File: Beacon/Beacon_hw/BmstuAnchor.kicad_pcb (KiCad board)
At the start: 2 copper layers, 62 x 60 mm, 46 parts, among them U1 MCP1700T-3002E/TT

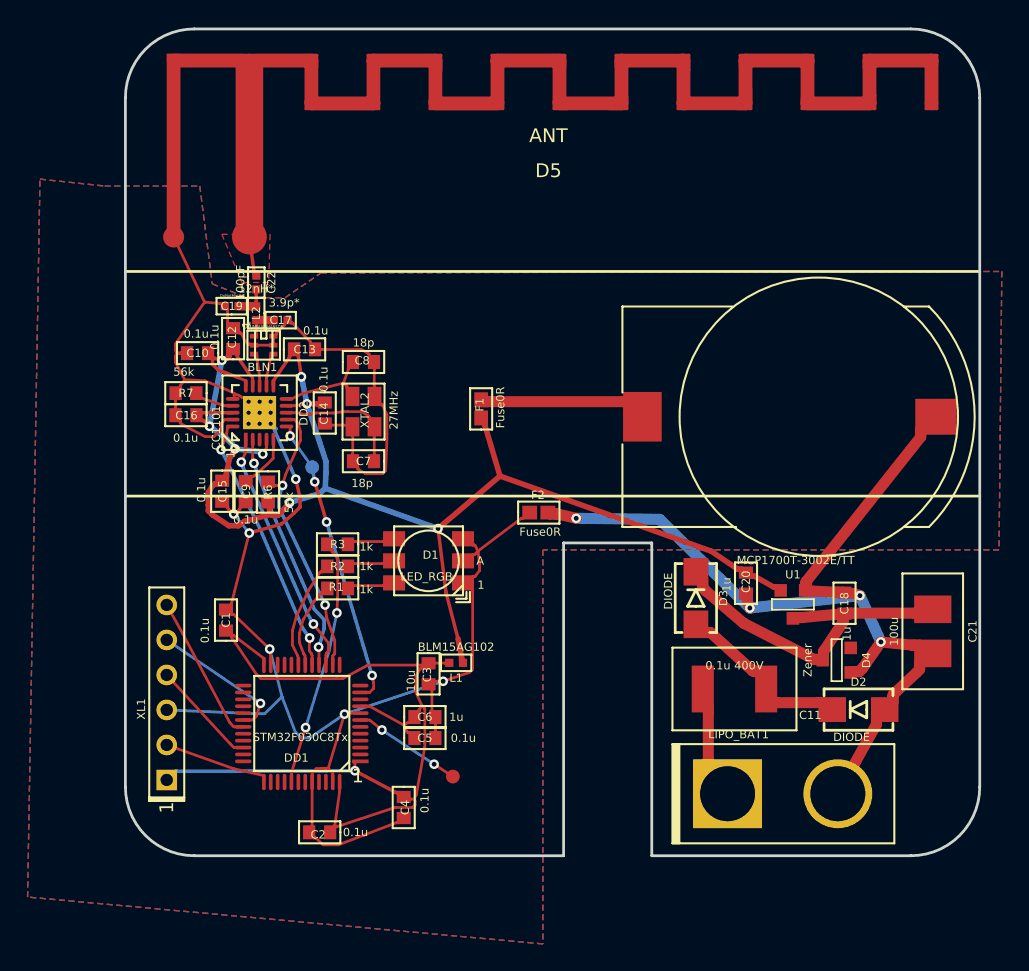
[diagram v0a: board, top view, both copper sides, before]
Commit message: +axp library *beaco pcb upd
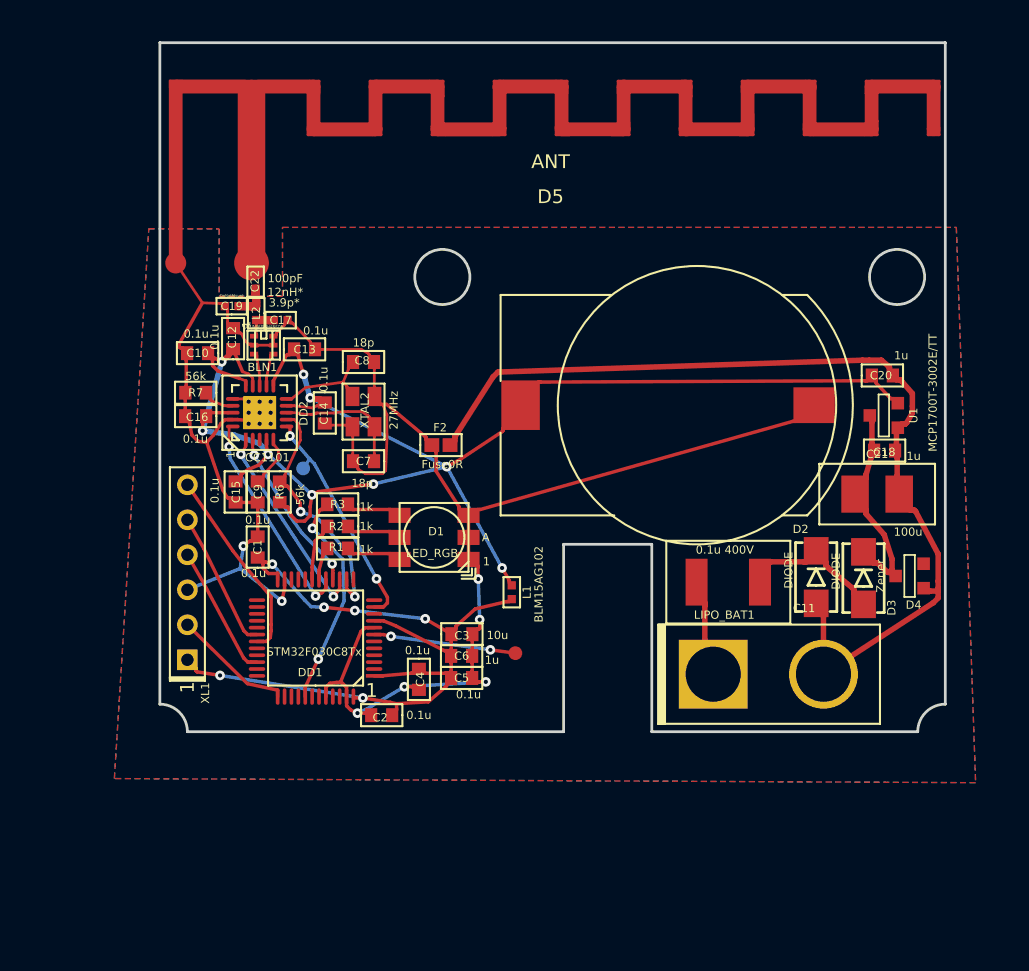
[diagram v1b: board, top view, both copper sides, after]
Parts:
- removed F1: Fuse0R, Resistors:RES_0603_FUSE
- moved C20 18.0 mm to (154.9, 125.1), turned to 0 degrees
- moved U1 15.2 mm to (155.0, 128.0), turned to 270 degrees
- moved D3 12.3 mm to (153.6, 139.9)
- moved C18 11.5 mm to (155.1, 130.6), turned to 0 degrees
- moved C21 10.7 mm to (154.6, 133.8), turned to 0 degrees
- moved D2 10.1 mm to (150.1, 139.8), turned to 270 degrees
- moved TP2 10.0 mm to (128.3, 145.3)
- moved C2 9.62 mm to (118.6, 149.8)
- moved C4 9.36 mm to (121.3, 147.2)
- moved B1 8.88 mm to (141.5, 127.3)
- moved XL1 8.85 mm to (104.5, 145.8)
- moved LIPO_BAT1 8.74 mm to (142.7, 146.8)
- moved F2 8.63 mm to (122.9, 130.2)
- moved D4 8.08 mm to (156.9, 139.7)
- moved C11 7.77 mm to (143.8, 140.1)
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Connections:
- B1 pad A: /BAT_+3V -> +3V
- B1 pad C: GND -> GNDS
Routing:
- net /BAT_+3V: track 12.3 -> 0.00 mm
- net Net-(C18-Pad1): track 25.8 -> 16.1 mm
- net GNDS: track 163.7 -> 154.3 mm, vias 6 -> 7
- net MCU_PWR: track 70.3 -> 61.6 mm, vias 1 -> 6
- net +3V: track 108.1 -> 116.2 mm, vias 8 -> 9
- net /CC_MISO: track 17.6 -> 12.0 mm
- net /CC_GDO0: track 21.5 -> 17.0 mm, vias 4 -> 2
- net /LED_R: track 6.34 -> 2.41 mm
- net /LED_G: track 8.01 -> 4.23 mm
- net /UART_RX: track 10.8 -> 14.2 mm
- net /CC_MOSI: track 19.3 -> 15.9 mm
- net /CC_SCK: track 18.0 -> 14.9 mm
- net /CC_CS: track 20.9 -> 17.9 mm
- net Net-(DD1-Pad7): track 7.98 -> 10.3 mm
- net Net-(C11-Pad1): track 13.1 -> 10.8 mm
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- removed copper zone on F.Cu, net Net-(C22-Pad1)
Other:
- board size 62 x 60 mm -> 57 x 50 mm
- net class Default: via_dia 0.8 -> 0.7; via_drill 0.4 -> 0.3
- rule pad_to_mask_clearance: 0.2 -> 0.1
